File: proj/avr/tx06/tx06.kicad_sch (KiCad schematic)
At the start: 3 parts, among them J1 Conn_02x10_Counter_Clockwise, J2 USB_C_Receptacle_USB2.0_14P, U1 ATtiny1606-M

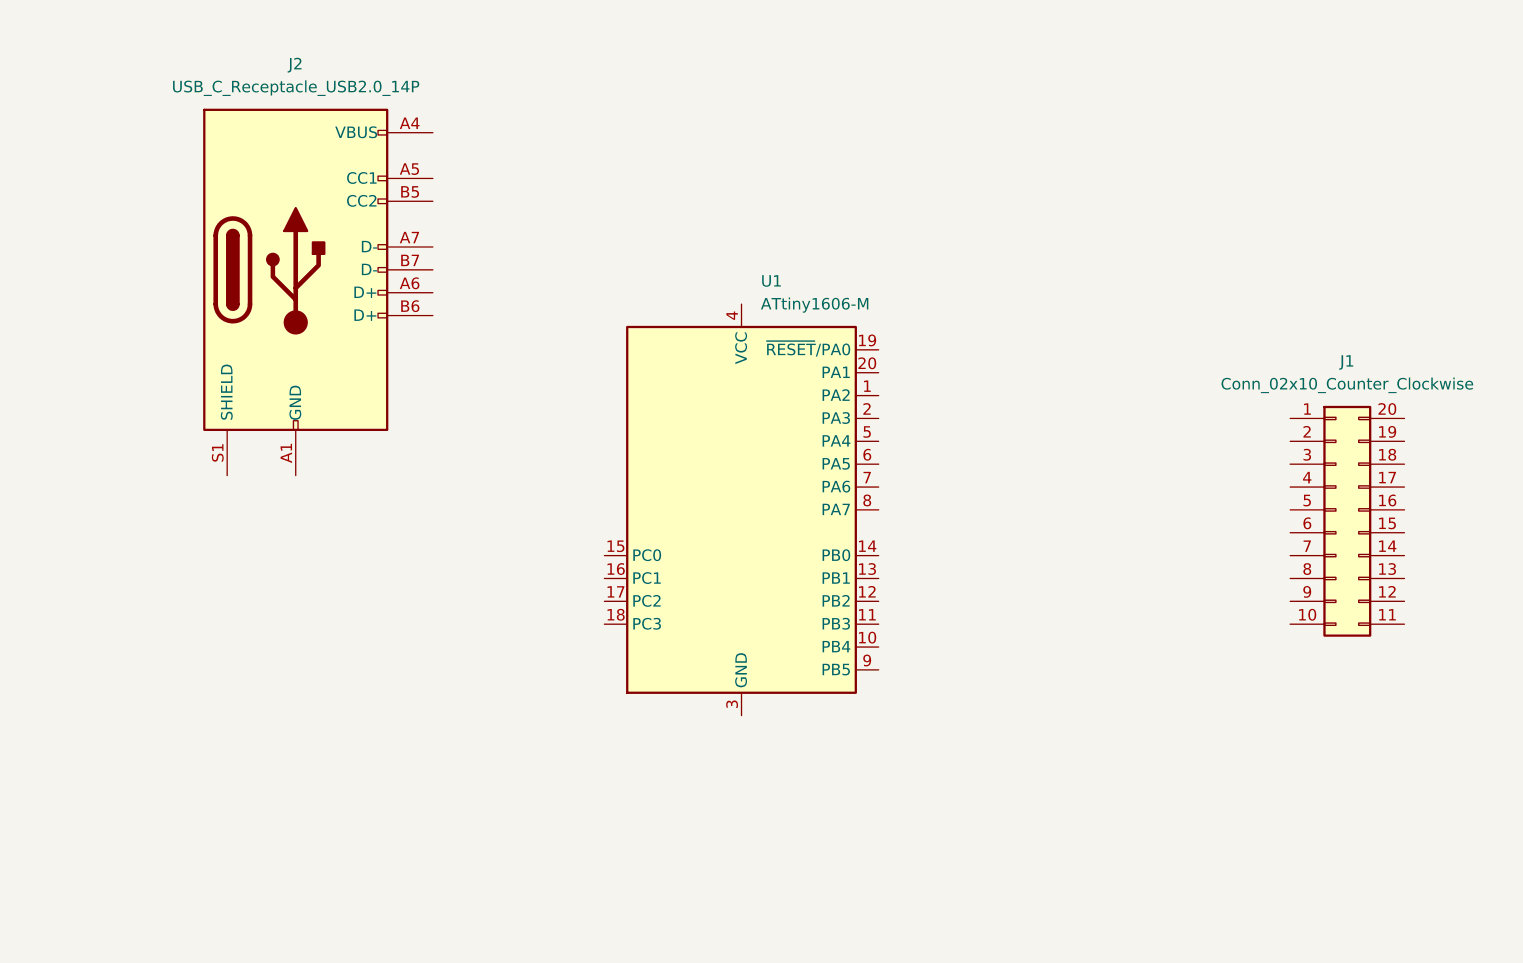
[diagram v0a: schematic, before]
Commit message: -
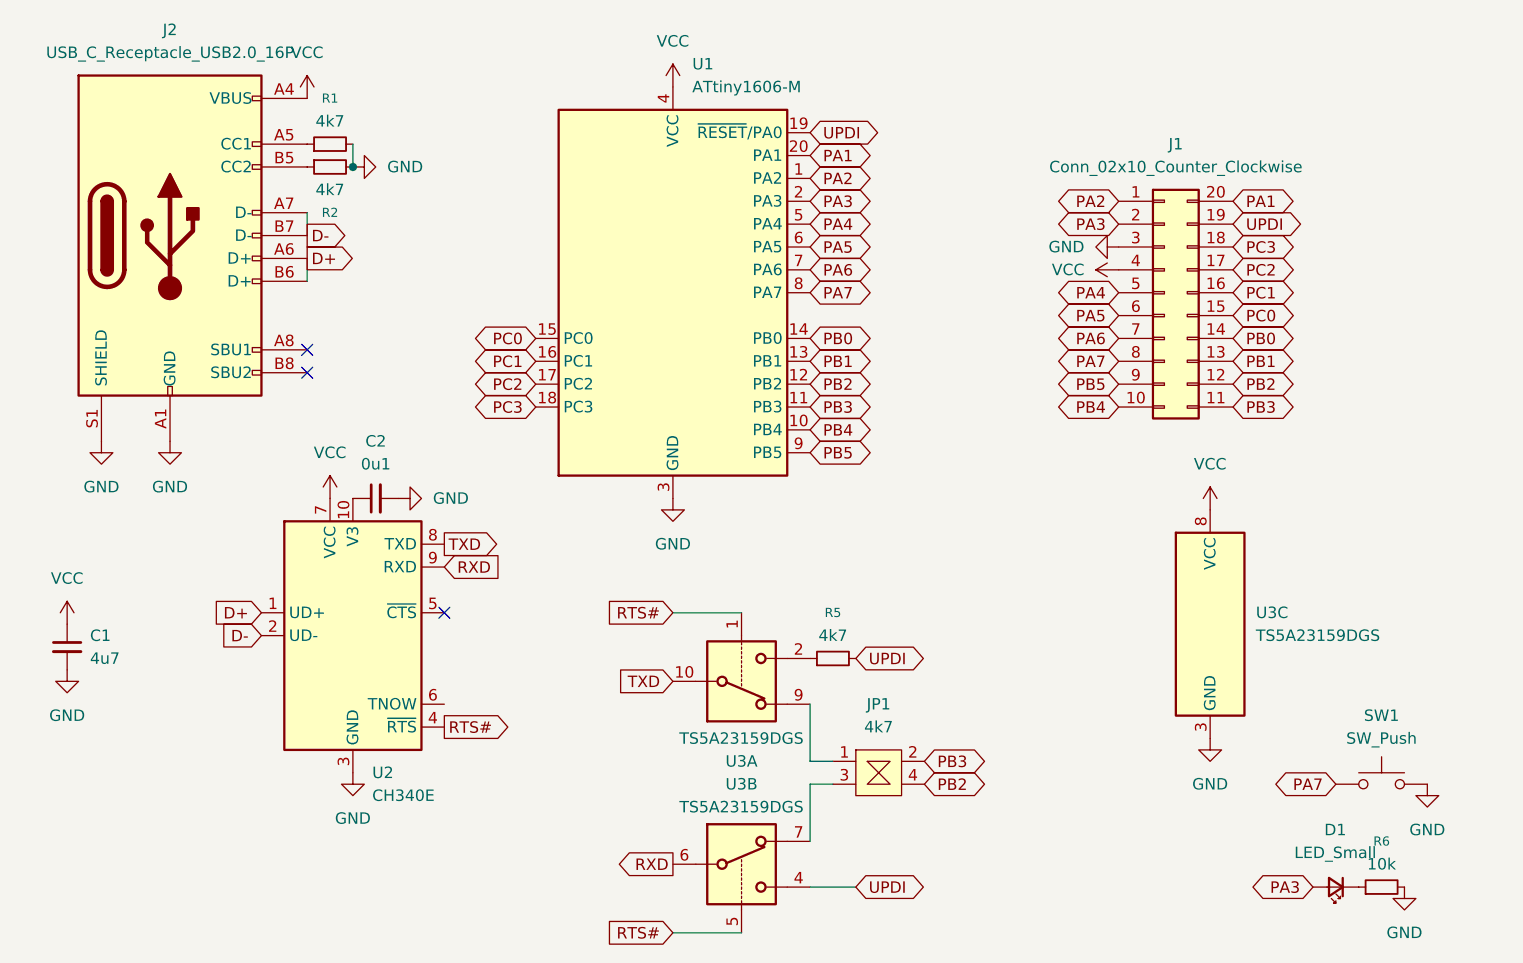
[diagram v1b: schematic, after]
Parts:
- removed J2: USB_C_Receptacle_USB2.0_14P, Library:USB-C, symbol Connector:USB_C_Receptacle_USB2.0_14P
- added C1: 4u7, Capacitor_SMD:C_0603_1608Metric, symbol Device:C_Small
- added C2: 0u1, Capacitor_SMD:C_0603_1608Metric, symbol Device:C_Small
- added D1: LED_Small, LED_SMD:LED_0603_1608Metric, symbol Device:LED_Small
- added J2: USB_C_Receptacle_USB2.0_16P, Connector_USB:USB_C_Receptacle_GCT_USB4105-xx-A_16P_TopMnt_Horizontal, symbol Connector:USB_C_Receptacle_USB2.0_16P
- added JP1: 4k7, Library:pokayoke_1608, symbol Library:pokayoke
- added R1, R2, R5: 4k7, Resistor_SMD:R_0603_1608Metric, symbol Device:R_Small
- added R6: 10k, Resistor_SMD:R_0603_1608Metric, symbol Device:R_Small
- added SW1: SW_Push, Library:alps-skrp, symbol Switch:SW_Push
- added U2: CH340E, Package_SO:MSOP-10_3x3mm_P0.5mm, symbol Interface_USB:CH340E
- added U3: TS5A23159DGS, Package_SO:VSSOP-10_3x3mm_P0.5mm, symbol Analog_Switch:TS5A23159DGS
- J1: footprint Package_DIP:DIP-20_W7.62mm -> Package_DIP:DIP-20_W7.62mm_Socket
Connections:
- net PA2: now reaches U1.1 (PA2)
- net PA2: now also J1.1 (Pin_1)
- net PB4: now reaches U1.10 (PB4)
- net PB4: now also J1.10 (Pin_10)
- net PB3: now reaches U1.11 (PB3)
- net PB3: now also J1.11 (Pin_11), JP1.2
- net PB2: now reaches U1.12 (PB2)
- net PB2: now also J1.12 (Pin_12), JP1.4
- net PB1: now reaches U1.13 (PB1)
- net PB1: now also J1.13 (Pin_13)
- net PB0: now reaches U1.14 (PB0)
- net PB0: now also J1.14 (Pin_14)
- net PC0: now reaches U1.15 (PC0)
- net PC0: now also J1.15 (Pin_15)
- net PC1: now reaches U1.16 (PC1)
- net PC1: now also J1.16 (Pin_16)
- net PC2: now reaches U1.17 (PC2)
- net PC2: now also J1.17 (Pin_17)
- net PC3: now reaches U1.18 (PC3)
- net PC3: now also J1.18 (Pin_18)
- net UPDI: now reaches U1.19 (~{RESET}/PA0)
- net UPDI: now also J1.19 (Pin_19), R5.2, U3.4
- net PA3: now reaches U1.2 (PA3)
- net PA3: now also J1.2 (Pin_2), D1.2 (A)
- net PA1: now reaches U1.20 (PA1)
- net PA1: now also J1.20 (Pin_20)
- net GND: now reaches U1.21 (GND), U1.3 (GND)
- net GND: now also J1.3 (Pin_3), C1.2, C2.2, J2.A1 (GND), J2.A12 (GND), J2.B1 (GND), J2.B12 (GND), J2.S1 (SHIELD), R1.2, R2.2, R6.2, SW1.2, U2.3 (GND), U3.3 (GND)
- net VCC: now reaches U1.4 (VCC)
- net VCC: now also J1.4 (Pin_4), C1.1, J2.A4 (VBUS), J2.A9 (VBUS), J2.B4 (VBUS), J2.B9 (VBUS), U2.7 (VCC), U3.8 (VCC)
- net PA4: now reaches U1.5 (PA4)
- net PA4: now also J1.5 (Pin_5)
- net PA5: now reaches U1.6 (PA5)
- net PA5: now also J1.6 (Pin_6)
- net PA6: now reaches U1.7 (PA6)
- net PA6: now also J1.7 (Pin_7)
- net PA7: now reaches U1.8 (PA7)
- net PA7: now also J1.8 (Pin_8), SW1.1
- net PB5: now reaches U1.9 (PB5)
- net PB5: now also J1.9 (Pin_9)
- new net: R5.1, U3.2
- new net: JP1.1, U3.9
- new net: JP1.3, U3.7
- new net: J2.A5 (CC1), R1.1
- new net: J2.B5 (CC2), R2.1
- new net: D1.1 (K), R6.1
- new net: C2.1, U2.10 (V3)
- new net D+: J2.A6 (D+), J2.B6 (D+), U2.1 (UD+)
- new net D-: J2.A7 (D-), J2.B7 (D-), U2.2 (UD-)
- new net RTS#: U2.4 (~{RTS}), U3.1, U3.5
- new net RXD: U2.9 (RXD), U3.6
- new net TXD: U2.8 (TXD), U3.10
- no-connect marks 0 -> 3
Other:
- moved on the sheet: J1, U1
